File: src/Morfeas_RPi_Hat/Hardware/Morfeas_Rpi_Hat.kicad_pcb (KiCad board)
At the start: 2 copper layers, 65 x 56 mm, 47 parts, among them J1 Power IN, J2 RPi_header, J3 CAN0_Power+, J4 CAN1_Power+, J5 RS_232, Q1 Q_PMOS_GDS, Q2 Q_PMOS_GDS, U1 DS3231, U2 TSR2-2450, U3 TLV70433, U4 SP3232, U5 24AA08, U6 MAX9611, U7 MAX9611

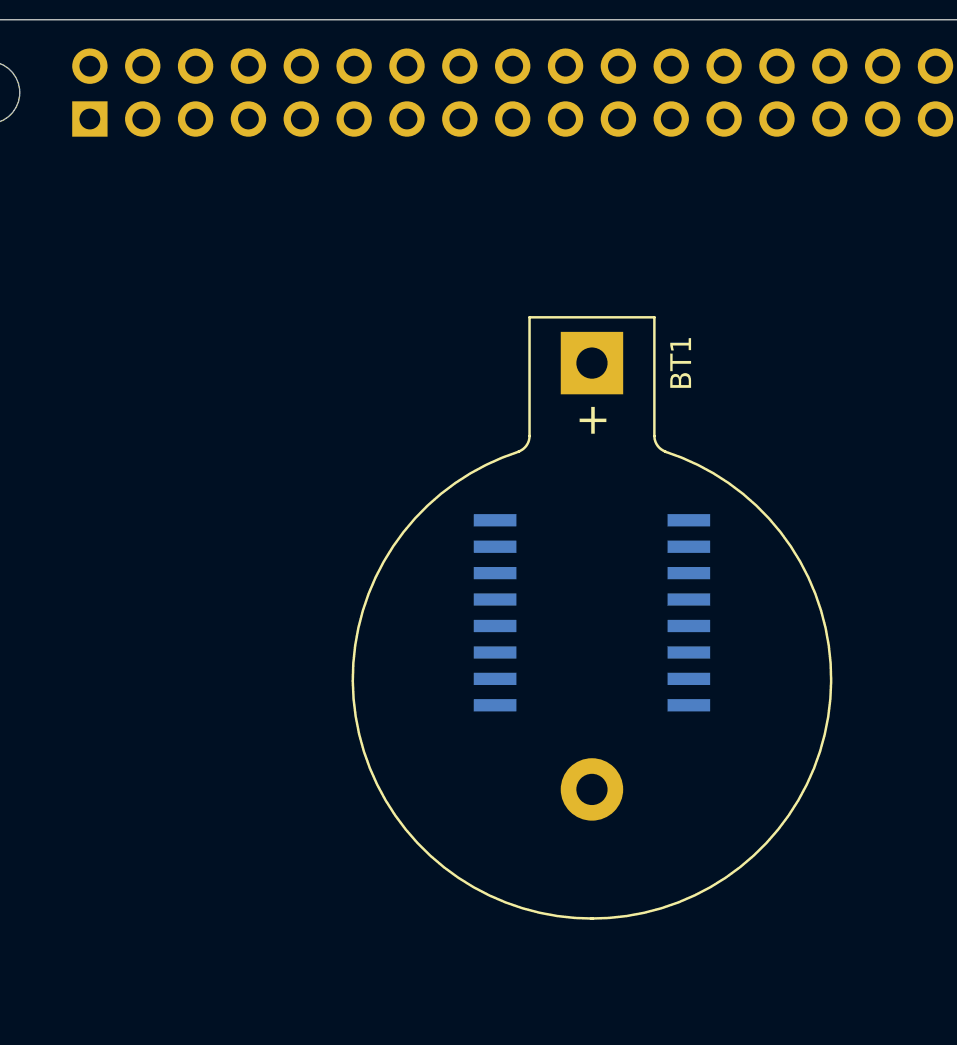
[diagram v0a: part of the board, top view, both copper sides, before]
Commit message: Update
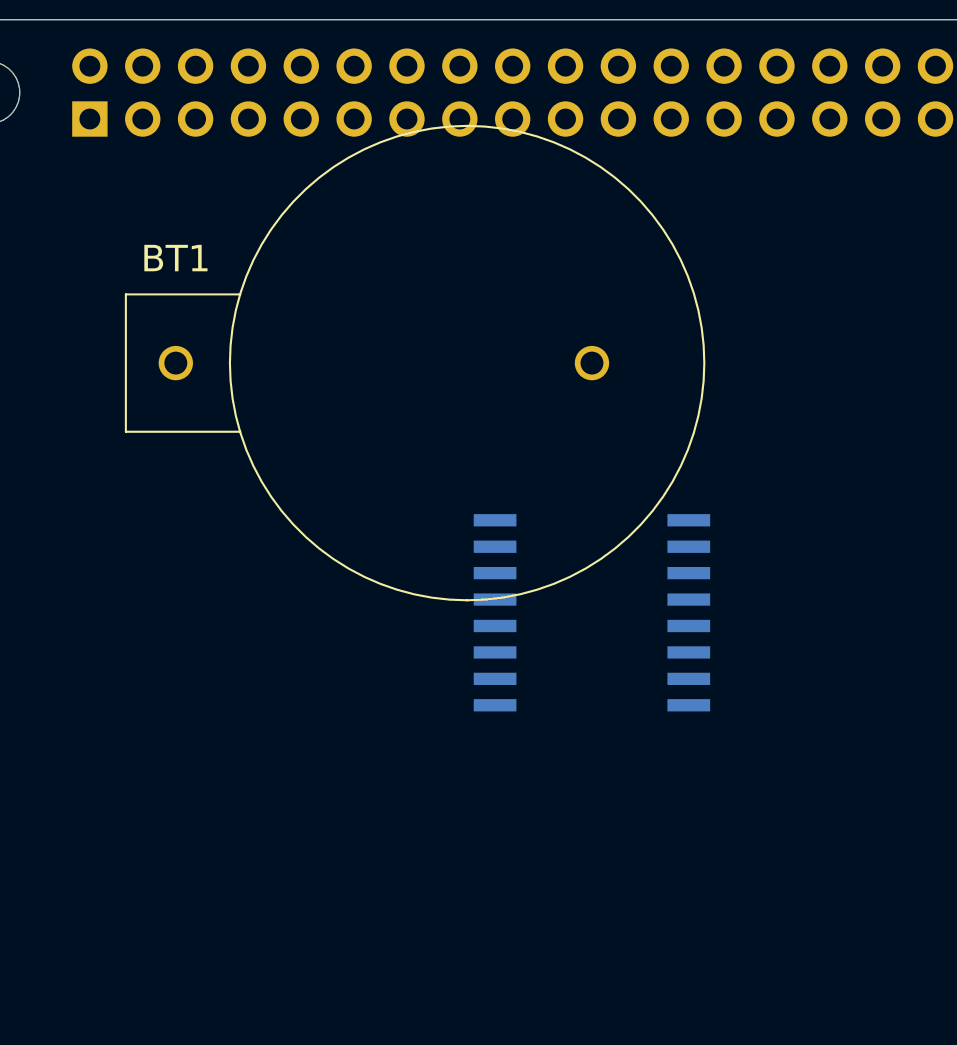
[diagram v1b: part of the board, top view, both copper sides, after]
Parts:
- BT1: footprint Battery:BatteryHolder_Keystone_103_1x20mm -> Morfeas_RPi_hat:CH252032LF
- Q1, Q2: value Q_PMOS_GDS -> SUM110P06
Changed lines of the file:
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@@
     (add_net +5V)
+  )
+  (module Morfeas_RPi_hat:CH252032LF (layer F.Cu)
+    (at 100.5 77.5 270)
+    (descr CH25-2032LF-1)
+    (tags "Undefined or Miscellaneous")
+    (fp_text reference BT1 (at -5 20) (layer F.SilkS)
+      (effects (font (size 1.27 1.27) (thickness 0.254)))
+    )
+    (fp_text value Battery_Cell (at 0 14.5 90) (layer F.SilkS) hide
+      (effects (font (size 1.27 1.27) (thickness 0.254)))
+    )
+    (fp_line (start -12.4 -6.4) (end 12.4 -6.4) (layer F.CrtYd) (width 0.1))
+    (fp_line (start 12.4 -6.4) (end 12.4 23.4) (layer F.CrtYd) (width 0.1))
+    (fp_line (start 12.4 23.4) (end -12.4 23.4) (layer F.CrtYd) (width 0.1))
+    (fp_line (start -12.4 23.4) (end -12.4 -6.4) (layer F.CrtYd) (width 0.1))
+    (fp_line (start -11.4 6) (end -11.4 6) (layer F.Fab) (width 0.2))
+    (fp_line (start 11.4 6) (end 11.4 6) (layer F.Fab) (width 0.2))
+    (fp_line (start -3.3 16.9) (end -3.3 22.4) (layer F.Fab) (width 0.2))
+    (fp_line (start -3.3 22.4) (end 3.3 22.4) (layer F.Fab) (width 0.2))
+    (fp_line (start 3.3 22.4) (end 3.3 16.9) (layer F.Fab) (width 0.2))
+    (fp_line (start -11.4 6) (end -11.4 6) (layer F.SilkS) (width 0.1))
+    (fp_line (start 11.4 6) (end 11.4 6) (layer F.SilkS) (width 0.1))
+    (fp_line (start -3.3 16.9) (end -3.3 22.4) (layer F.SilkS) (width 0.1))
+    (fp_line (start -3.3 22.4) (end 3.3 22.4) (layer F.SilkS) (width 0.1))
+    (fp_line (start 3.3 22.4) (end 3.3 16.9) (layer F.SilkS) (width 0.1))
+    (fp_arc (start 0 6) (end -11.4 6) (angle -180) (layer F.Fab) (width 0.2))
+    (fp_arc (start 0 6) (end 11.4 6) (angle -180) (layer F.Fab) (width 0.2))
+    (fp_arc (start 0 6) (end -11.4 6) (angle -180) (layer F.SilkS) (width 0.1))
+    (fp_arc (start 0 6) (end 11.4 6) (angle -180) (layer F.SilkS) (width 0.1))
+    (pad 1 thru_hole circle (at 0 0 270) (size 1.65 1.65) (drill 1.1) (layers *.Cu *.Mask)
+      (net 2 "Net-(BT1-Pad1)"))
+    (pad 2 thru_hole circle (at 0 20 270) (size 1.65 1.65) (drill 1.1) (layers *.Cu *.Mask)
+      (net 1 GND))
+    (model ${KIPRJMOD}/Project's_libs/STEP/CH25-2032LF_approx.step
+      (offset (xyz 0 -5.99948 0))
+      (scale (xyz 1 1 1))
+      (rotate (xyz 0 0 180))
+    )
   )
   (module Morfeas_RPi_hat:TLV70433DBVT (layer F.Cu)
@@
       (effects (font (size 1 1) (thickness 0.15)))
     )
-    (fp_text value Q_PMOS_GDS (at 0 6.65) (layer F.Fab)
+    (fp_text value SUM110P06 (at 0 6.65) (layer F.Fab)
       (effects (font (size 1 1) (thickness 0.15)))
     )
@@
       (effects (font (size 1 1) (thickness 0.15)))
     )
-    (fp_text value Q_PMOS_GDS (at 0 6.65) (layer F.Fab)
+    (fp_text value SUM110P06 (at 0 6.65) (layer F.Fab)
       (effects (font (size 1 1) (thickness 0.15)))
     )
@@
       (at (xyz 0 0 0))
       (scale (xyz 1 1 1))
-      (rotate (xyz 0 0 0))
-    )
-  )
-  (module Battery:BatteryHolder_Keystone_103_1x20mm (layer F.Cu)
-    (at 100.5 77.5 270)
-    (descr http://www.keyelco.com/product-pdf.cfm?p=719)
-    (tags "Keystone type 103 battery holder")
-    (fp_text reference BT1 (at 0 -4.3 90) (layer F.SilkS)
-      (effects (font (size 1 1) (thickness 0.15)))
-    )
-    (fp_text value Battery_Cell (at 15 13 90) (layer F.Fab)
-      (effects (font (size 1 1) (thickness 0.15)))
-    )
-    (fp_text user + (at 2.75 0 90) (layer F.SilkS)
-      (effects (font (size 1.5 1.5) (thickness 0.15)))
-    )
-    (fp_text user %R (at 0 0 90) (layer F.Fab)
-      (effects (font (size 1 1) (thickness 0.15)))
-    )
-    (fp_arc (start 15.2 0) (end 4.01 3.6) (angle -162.5) (layer F.CrtYd) (width 0.05))
-    (fp_arc (start 15.2 0) (end 4.01 -3.6) (angle 162.5) (layer F.CrtYd) (width 0.05))
-    (fp_arc (start 3.5 3.8) (end 3.5 3.25) (angle 70) (layer F.CrtYd) (width 0.05))
-    (fp_arc (start 3.5 -3.8) (end 3.5 -3.25) (angle -70) (layer F.CrtYd) (width 0.05))
-    (fp_arc (start 15.2 0) (end 4.25 3.5) (angle -162.5) (layer F.SilkS) (width 0.12))
-    (fp_arc (start 3.5 3.8) (end 3.5 3) (angle 70) (layer F.SilkS) (width 0.12))
-    (fp_arc (start 15.2 0) (end 4.25 -3.5) (angle 162.5) (layer F.SilkS) (width 0.12))
-    (fp_arc (start 3.5 -3.8) (end 3.5 -3) (angle -70) (layer F.SilkS) (width 0.12))
-    (fp_arc (start 3.5 3.8) (end 3.5 2.9) (angle 70) (layer F.Fab) (width 0.1))
-    (fp_arc (start 15.2 0) (end 4.35 3.5) (angle -162.5) (layer F.Fab) (width 0.1))
-    (fp_arc (start 15.2 0) (end 4.35 -3.5) (angle 162.5) (layer F.Fab) (width 0.1))
-    (fp_arc (start 15.2 0) (end 5.2 1.3) (angle -180) (layer F.Fab) (width 0.1))
-    (fp_line (start -2.45 -3.25) (end 3.5 -3.25) (layer F.CrtYd) (width 0.05))
-    (fp_line (start -2.45 3.25) (end 3.5 3.25) (layer F.CrtYd) (width 0.05))
-    (fp_line (start -2.45 3.25) (end -2.45 -3.25) (layer F.CrtYd) (width 0.05))
-    (fp_line (start -2.2 -3) (end 3.5 -3) (layer F.SilkS) (width 0.12))
-    (fp_line (start -2.2 3) (end -2.2 -3) (layer F.SilkS) (width 0.12))
-    (fp_line (start -2.2 3) (end 3.5 3) (layer F.SilkS) (width 0.12))
-    (fp_arc (start 15.2 0) (end 9 1.3) (angle -170) (layer F.Fab) (width 0.1))
-    (fp_arc (start 15.2 0) (end 13.3 1.3) (angle -150) (layer F.Fab) (width 0.1))
-    (fp_line (start 23.5712 7.7216) (end 22.6568 6.8834) (layer F.Fab) (width 0.1))
-    (fp_line (start 23.5712 -7.7216) (end 22.6314 -6.858) (layer F.Fab) (width 0.1))
-    (fp_arc (start 15.2 0) (end 13.3 -1.3) (angle 150) (layer F.Fab) (width 0.1))
-    (fp_arc (start 15.2 0) (end 9 -1.3) (angle 170) (layer F.Fab) (width 0.1))
-    (fp_arc (start 15.2 0) (end 5.2 -1.3) (angle 180) (layer F.Fab) (width 0.1))
-    (fp_line (start 3.5306 -2.9) (end -1.7 -2.9) (layer F.Fab) (width 0.1))
-    (fp_line (start -1.7 2.9) (end 3.5306 2.9) (layer F.Fab) (width 0.1))
-    (fp_line (start -2.1 -2.5) (end -2.1 2.5) (layer F.Fab) (width 0.1))
-    (fp_line (start 0 1.3) (end 16.2 1.3) (layer F.Fab) (width 0.1))
-    (fp_line (start 16.2 -1.3) (end 0 -1.3) (layer F.Fab) (width 0.1))
-    (fp_arc (start 3.5 -3.8) (end 3.5 -2.9) (angle -70) (layer F.Fab) (width 0.1))
-    (fp_arc (start 16.2 0) (end 16.2 -1.3) (angle 180) (layer F.Fab) (width 0.1))
-    (fp_line (start 0 -1.3) (end 0 1.3) (layer F.Fab) (width 0.1))
-    (fp_arc (start -1.7 2.5) (end -2.1 2.5) (angle -90) (layer F.Fab) (width 0.1))
-    (fp_arc (start -1.7 -2.5) (end -2.1 -2.5) (angle 90) (layer F.Fab) (width 0.1))
-    (pad 2 thru_hole circle (at 20.49 0 270) (size 3 3) (drill 1.5) (layers *.Cu *.Mask)
-      (net 1 GND))
-    (pad 1 thru_hole rect (at 0 0 270) (size 3 3) (drill 1.5) (layers *.Cu *.Mask)
-      (net 2 "Net-(BT1-Pad1)"))
-    (model ${KISYS3DMOD}/Battery.3dshapes/BatteryHolder_Keystone_103_1x20mm.wrl
-      (at (xyz 0 0 0))
-      (scale (xyz 1 1 1))
